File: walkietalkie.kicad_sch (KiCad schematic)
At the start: 7 parts, among them SW2 SW_Push, U2 NRF24L01_Breakout

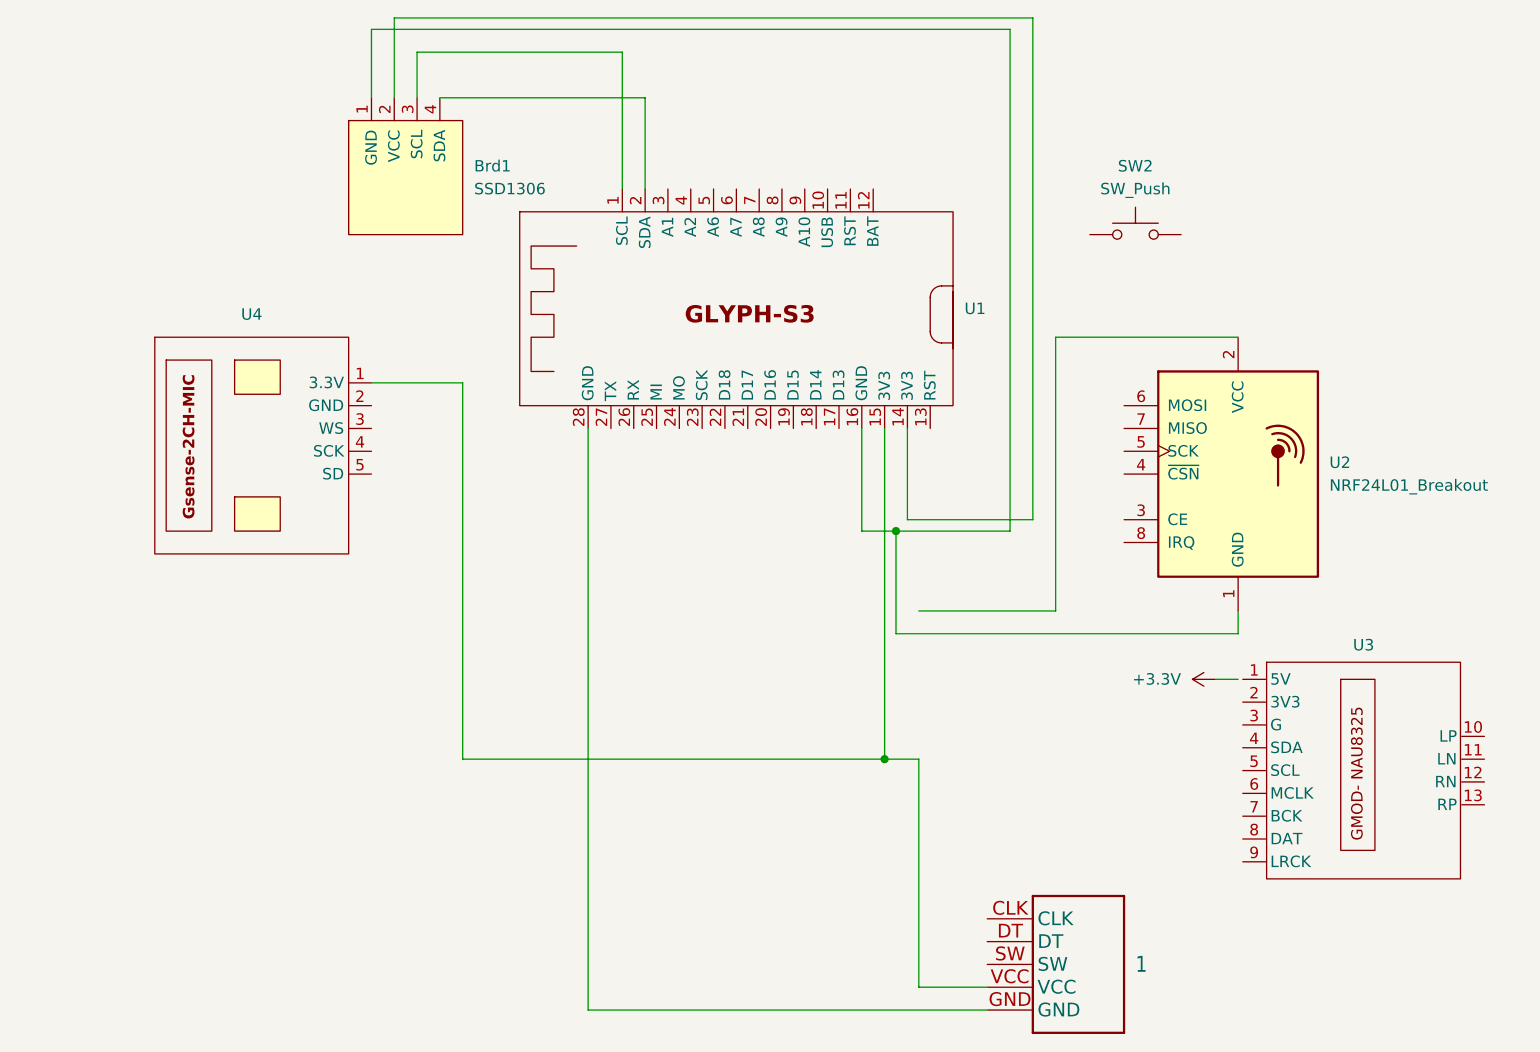
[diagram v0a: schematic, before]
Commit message: schematics done
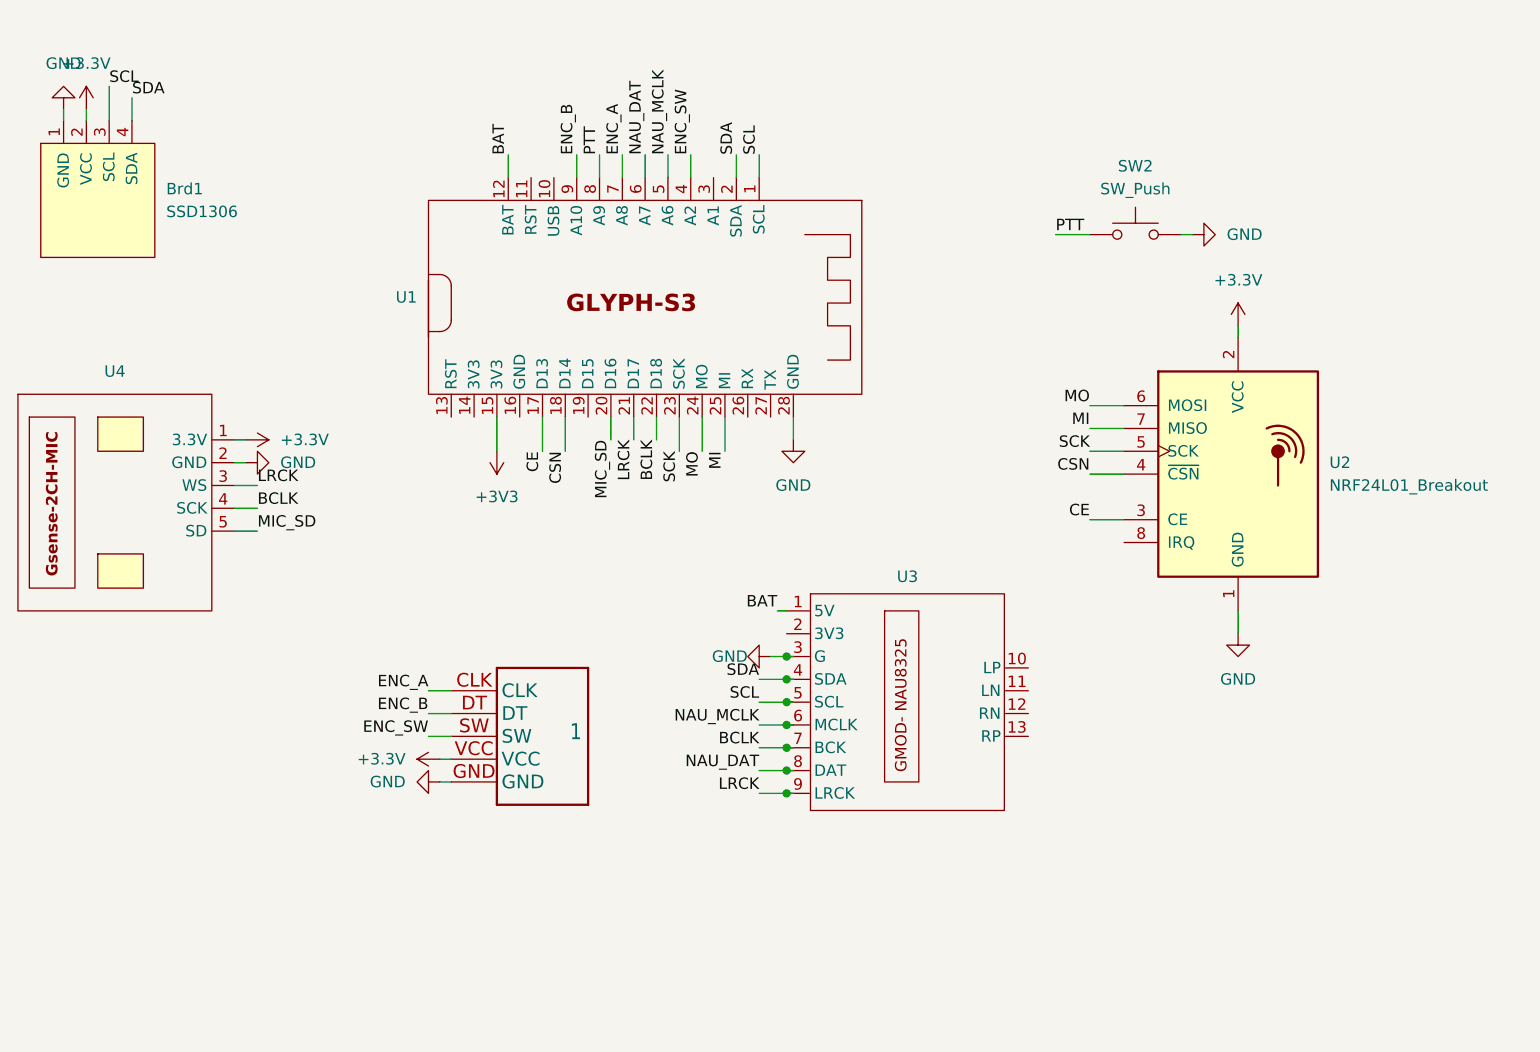
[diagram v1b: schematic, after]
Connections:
- net +3.3V: now also 1.VCC, Brd1.2 (VCC), U2.2 (VCC), U4.1 (3.3V)
- net SCL: now reaches Brd1.3 (SCL), U1.1 (SCL)
- net SCL: now also U3.5 (SCL)
- net BAT: now reaches U1.12 (BAT)
- net BAT: now also U3.1 (5V)
- net at U1.14 (3V3): no longer Brd1.2 (VCC)
- net GND: now reaches Brd1.1 (GND), U2.1 (GND)
- net GND: now also 1.GND, SW2.2, U1.28 (GND), U3.3 (G), U4.2 (GND); no longer U1.16 (GND)
- net CE: now reaches U1.17 (D13)
- net CE: now also U2.3 (CE)
- net CSN: now reaches U1.18 (D14)
- net CSN: now also U2.4 (~{CSN})
- net SDA: now reaches Brd1.4 (SDA), U1.2 (SDA)
- net SDA: now also U3.4 (SDA)
- net MIC_SD: now reaches U1.20 (D16)
- net MIC_SD: now also U4.5 (SD)
- net LRCK: now reaches U1.21 (D17)
- net LRCK: now also U3.9 (LRCK), U4.3 (WS)
- net BCLK: now reaches U1.22 (D18)
- net BCLK: now also U3.7 (BCK), U4.4 (SCK)
- net SCK: now reaches U1.23 (SCK)
- net SCK: now also U2.5 (SCK)
- net MO: now reaches U1.24 (MO)
- net MO: now also U2.6 (MOSI)
- net MI: now reaches U1.25 (MI)
- net MI: now also U2.7 (MISO)
- net ENC_SW: now reaches U1.4 (A2)
- net ENC_SW: now also 1.SW
- net NAU_MCLK: now reaches U1.5 (A6)
- net NAU_MCLK: now also U3.6 (MCLK)
- net NAU_DAT: now reaches U1.6 (A7)
- net NAU_DAT: now also U3.8 (DAT)
- net ENC_A: now reaches U1.7 (A8)
- net ENC_A: now also 1.CLK
- net PTT: now reaches U1.8 (A9)
- net PTT: now also SW2.1
- net ENC_B: now reaches U1.9 (A10)
- net ENC_B: now also 1.DT
- new net +3V3: U1.15 (3V3)
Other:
- moved on the sheet: 1, Brd1, U1, U3, U4
